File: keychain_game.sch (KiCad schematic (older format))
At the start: 28 parts, among them J1 Conn_02x03_Counter_Clockwise, J2 Conn_01x02, SW1 SW_MEC_5G, U1 MIC5205-2.5, U2 SN74HC595DR, U4 ATTINY13A-MMF

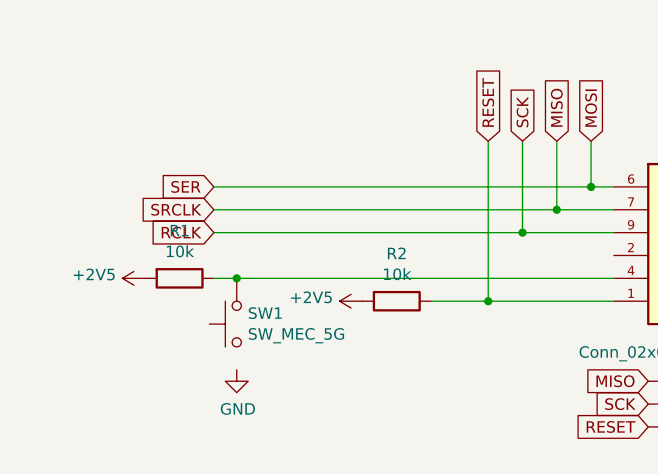
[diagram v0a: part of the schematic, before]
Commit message: finished board
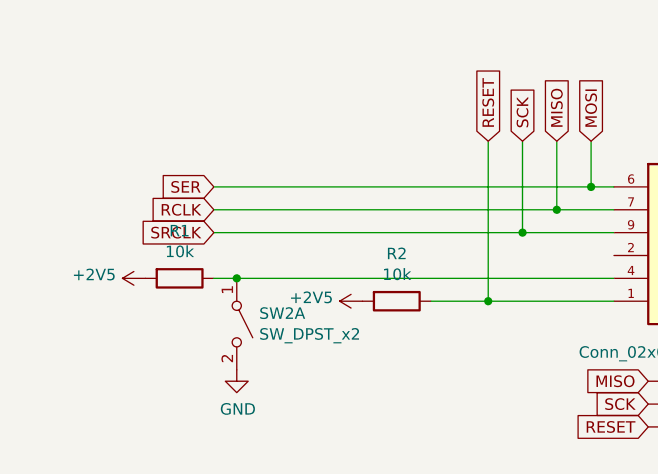
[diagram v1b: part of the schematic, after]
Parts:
- removed SW1: SW_MEC_5G, Button_Switch_SMD:SW_SPST_B3U-1000P, symbol Switch:SW_MEC_5G
- added SW2: SW_DPST_x2, Button_Switch_SMD:SW_SPST_B3U-1000P, symbol Switch:SW_DPST_x2
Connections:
- net GND: now also SW2.2 (B)
- net MISO: now also U2.12 (RCLK); no longer U2.11 (SRCLK)
- net at R1.1, U4.4 (PB4(ADC2/PCINT4)): now also SW2.1 (A)
- net RCLK renamed SCK
- net SCK: now also U2.11 (SRCLK); no longer U2.12 (RCLK)
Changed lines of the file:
@@
 Text GLabel 3400 2050 0    50   Input ~ 0
 RCLK
+Text GLabel 1900 4250 0    50   Input ~ 0
+RCLK
 Text GLabel 1900 4350 0    50   Input ~ 0
-RCLK
-Text GLabel 1900 4250 0    50   Input ~ 0
 SRCLK
 Text GLabel 1900 4150 0    50   Input ~ 0
@@
 F 3 "" H 1600 4550 50  0001 C CNN
 	1    1600 4550
-	0    -1   -1   0
-$EndComp
-$Comp
-L Switch:SW_MEC_5G SW1
-U 1 1 5B7E7332
-P 2000 4750
-F 0 "SW1" V 2046 4702 50  0000 R CNN
-F 1 "SW_MEC_5G" V 1955 4702 50  0000 R CNN
-F 2 "Button_Switch_SMD:SW_SPST_B3U-1000P" H 2000 4950 50  0001 C CNN
-F 3 "http://www.apem.com/int/index.php?controller=attachment&id_attachment=488" H 2000 4950 50  0001 C CNN
-	1    2000 4750
 	0    -1   -1   0
 $EndComp
@@
 	1    0    0    -1
 $EndComp
+$Comp
+L Switch:SW_DPST_x2 SW2
+U 1 1 5B8A0B61
+P 2000 4750
+F 0 "SW2" V 1954 4848 50  0000 L CNN
+F 1 "SW_DPST_x2" V 2045 4848 50  0000 L CNN
+F 2 "Button_Switch_SMD:SW_SPST_B3U-1000P" H 2000 4750 50  0001 C CNN
+F 3 "" H 2000 4750 50  0001 C CNN
+	1    2000 4750
+	0    1    1    0
+$EndComp
 $EndSCHEMATC
